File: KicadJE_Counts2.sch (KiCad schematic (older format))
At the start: 91 parts, among them J403 Out 1, J404 In_1, J405 Out 2, J406 In 2, J407 Out 1 Final, J408 Out 2 Final, U401 TL072, U402 TL072

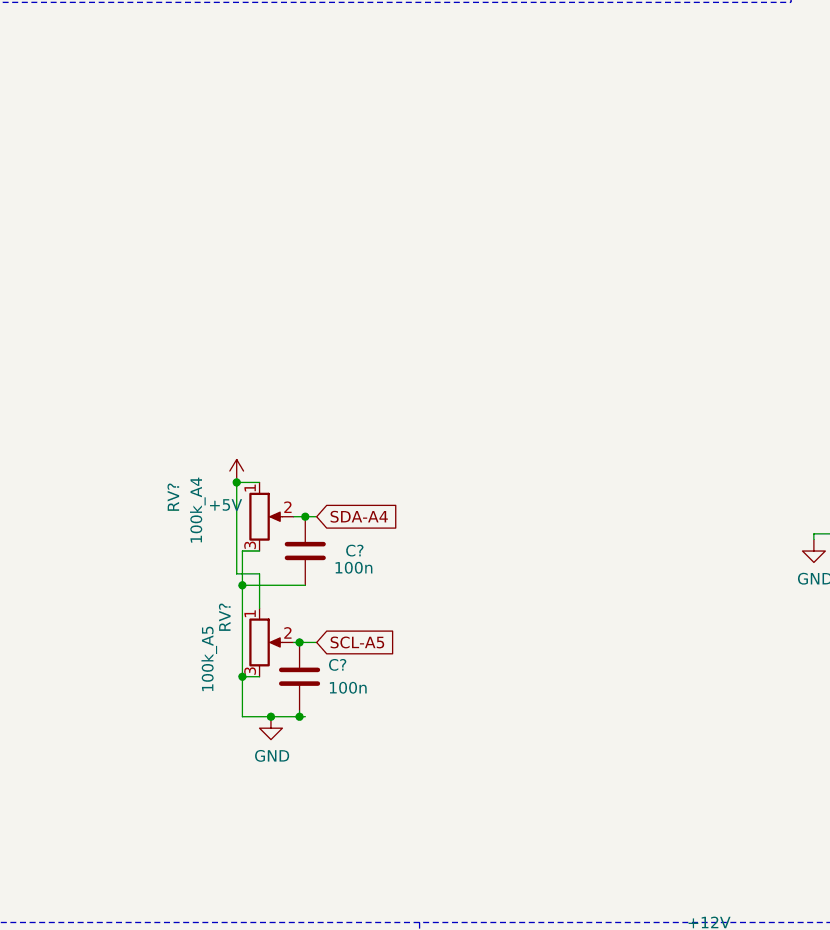
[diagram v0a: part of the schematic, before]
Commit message: Update KicadJE_Counts2.sch
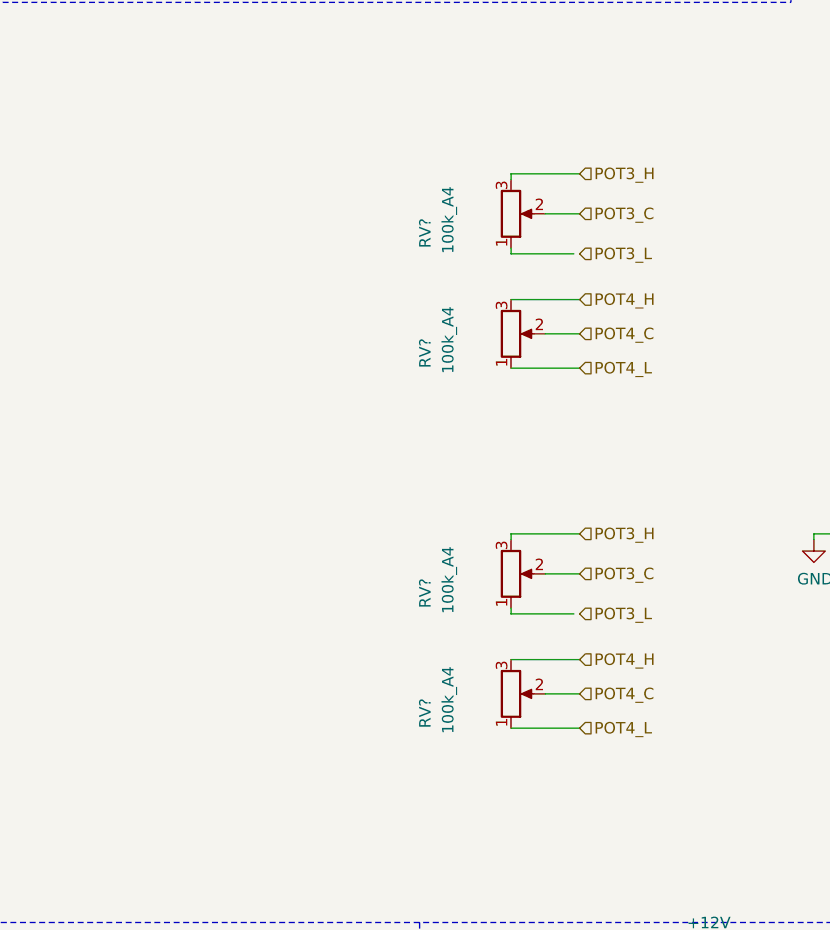
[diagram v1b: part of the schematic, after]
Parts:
- removed C? (x2): 100n, Capacitor_SMD:C_0805_2012Metric_Pad1.15x1.40mm_HandSolder, symbol Device:C
- removed RV?: 100k_A5, Potentiometer_THT:Potentiometer_China_RK09_Single_Vertical_AJ, symbol Device:R_POT
- added RV? (x3): 100k_A4, Potentiometer_THT:Potentiometer_China_RK09_Single_Vertical_AJ, symbol Device:R_POT
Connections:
- net SDA-A4 is gone; now on net POT3_C: RV?.2
- net +5V: no longer RV?.1
- net GND: no longer RV?.3
- net POT3_C: now also RV?.3, RV?.2, RV?.3
- net POT4_C: now also RV?.2, RV?.2, RV?.3, RV?.3
- net POT4_L: now also RV?.1, RV?.1
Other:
- moved on the sheet: RV?
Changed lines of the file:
@@
 Wire Wire Line
 	3800 6100 3875 6100
-Text GLabel 2100 4700 2    50   Input ~ 0
-SCL-A5
-Text GLabel 2100 4150 2    50   Input ~ 0
-SDA-A4
 $Comp
 L Device:R_POT RV?
 U 1 1 5F13A9C4
-P 1850 4150
+P 2950 4400
 AR Path="/5F13A9C4" Ref="RV?"  Part="1"
 AR Path="/5D60ED9A/5F13A9C4" Ref="RV?"  Part="1"
-F 0 "RV?" V 1475 4300 50  0000 R CNN
-F 1 "100k_A4" V 1575 4325 50  0000 R CNN
-F 2 "Potentiometer_THT:Potentiometer_China_RK09_Single_Vertical_AJ" H 1850 4150 50  0001 C CNN
-F 3 "~" H 1850 4150 50  0001 C CNN
-	1    1850 4150
-	1    0    0    -1
-$EndComp
-Wire Wire Line
-	2000 4150 2050 4150
-$Comp
-L Device:R_POT RV?
-U 1 1 5F13A9CB
-P 1850 4700
-AR Path="/5F13A9CB" Ref="RV?"  Part="1"
-AR Path="/5D60ED9A/5F13A9CB" Ref="RV?"  Part="1"
-F 0 "RV?" V 1700 4875 50  0000 R CNN
-F 1 "100k_A5" V 1625 4775 50  0000 R CNN
-F 2 "Potentiometer_THT:Potentiometer_China_RK09_Single_Vertical_AJ" H 1850 4700 50  0001 C CNN
-F 3 "~" H 1850 4700 50  0001 C CNN
-	1    1850 4700
-	1    0    0    -1
-$EndComp
-Wire Wire Line
-	2000 4700 2025 4700
-Wire Wire Line
-	1750 4400 1750 4000
-Wire Wire Line
-	1750 4000 1850 4000
-Wire Wire Line
-	1775 4850 1850 4850
-$Comp
-L power:GND #PWR?
-U 1 1 5F13A9D5
-P 1900 5025
-AR Path="/5F13A9D5" Ref="#PWR?"  Part="1"
-AR Path="/5D60ED9A/5F13A9D5" Ref="#PWR?"  Part="1"
-F 0 "#PWR?" H 1900 4775 50  0001 C CNN
-F 1 "GND" H 1905 4852 50  0000 C CNN
-F 2 "" H 1900 5025 50  0001 C CNN
-F 3 "" H 1900 5025 50  0001 C CNN
-	1    1900 5025
-	1    0    0    -1
-$EndComp
-$Comp
-L power:+5V #PWR?
-U 1 1 5F13A9DB
-P 1750 4000
-AR Path="/5F13A9DB" Ref="#PWR?"  Part="1"
-AR Path="/5D60ED9A/5F13A9DB" Ref="#PWR?"  Part="1"
-F 0 "#PWR?" H 1750 3850 50  0001 C CNN
-F 1 "+5V" H 1700 3900 50  0000 C CNN
-F 2 "" H 1750 4000 50  0001 C CNN
-F 3 "" H 1750 4000 50  0001 C CNN
-	1    1750 4000
-	1    0    0    -1
-$EndComp
-Connection ~ 1750 4000
-$Comp
-L Device:C C?
-U 1 1 5F13A9E2
-P 2025 4850
-AR Path="/5F13A9E2" Ref="C?"  Part="1"
-AR Path="/5D60ED9A/5F13A9E2" Ref="C?"  Part="1"
-F 0 "C?" H 2150 4900 50  0000 L CNN
-F 1 "100n" H 2150 4800 50  0000 L CNN
-F 2 "Capacitor_SMD:C_0805_2012Metric_Pad1.15x1.40mm_HandSolder" H 2063 4700 50  0001 C CNN
-F 3 "~" H 2025 4850 50  0001 C CNN
-	1    2025 4850
-	1    0    0    -1
-$EndComp
-Connection ~ 2025 4700
-Wire Wire Line
-	2025 4700 2100 4700
-Wire Wire Line
-	1775 4850 1775 5025
-Wire Wire Line
-	1775 5025 1900 5025
-Wire Wire Line
-	2025 5025 2025 5000
-Connection ~ 1900 5025
-Wire Wire Line
-	1900 5025 2025 5025
-$Comp
-L Device:C C?
-U 1 1 5F13A9EF
-P 2050 4300
-AR Path="/5F13A9EF" Ref="C?"  Part="1"
-AR Path="/5D60ED9A/5F13A9EF" Ref="C?"  Part="1"
-F 0 "C?" H 2225 4300 50  0000 L CNN
-F 1 "100n" H 2175 4225 50  0000 L CNN
-F 2 "Capacitor_SMD:C_0805_2012Metric_Pad1.15x1.40mm_HandSolder" H 2088 4150 50  0001 C CNN
-F 3 "~" H 2050 4300 50  0001 C CNN
-	1    2050 4300
-	1    0    0    -1
-$EndComp
-Connection ~ 2050 4150
-Wire Wire Line
-	2050 4150 2100 4150
-Wire Wire Line
-	2050 5025 2025 5025
-Connection ~ 2025 5025
-Wire Wire Line
-	1850 4550 1850 4400
-Wire Wire Line
-	1850 4400 1750 4400
-Wire Wire Line
-	1850 4300 1775 4300
-Wire Wire Line
-	1775 4300 1775 4450
-Connection ~ 1775 4850
-Wire Wire Line
-	2050 4450 1775 4450
-Connection ~ 1775 4450
-Wire Wire Line
-	1775 4450 1775 4850
+F 0 "RV?" V 2575 4550 50  0000 R CNN
+F 1 "100k_A4" V 2675 4575 50  0000 R CNN
+F 2 "Potentiometer_THT:Potentiometer_China_RK09_Single_Vertical_AJ" H 2950 4400 50  0001 C CNN
+F 3 "~" H 2950 4400 50  0001 C CNN
+	1    2950 4400
+	1    0    0    1
+$EndComp
 $Comp
 L Device:C C?
@@
 Wire Notes Line
 	600  1900 4175 1900
+Text HLabel 3250 4225 2    50   Input ~ 0
+POT3_H
+Text HLabel 3250 4400 2    50   Input ~ 0
+POT3_C
+Text HLabel 3250 4575 2    50   Input ~ 0
+POT3_L
+Text HLabel 3250 4775 2    50   Input ~ 0
+POT4_H
+Text HLabel 3250 4925 2    50   Input ~ 0
+POT4_C
+Text HLabel 3250 5075 2    50   Input ~ 0
+POT4_L
+$Comp
+L Device:R_POT RV?
+U 1 1 5F31783B
+P 2950 4925
+AR Path="/5F31783B" Ref="RV?"  Part="1"
+AR Path="/5D60ED9A/5F31783B" Ref="RV?"  Part="1"
+F 0 "RV?" V 2575 5075 50  0000 R CNN
+F 1 "100k_A4" V 2675 5100 50  0000 R CNN
+F 2 "Potentiometer_THT:Potentiometer_China_RK09_Single_Vertical_AJ" H 2950 4925 50  0001 C CNN
+F 3 "~" H 2950 4925 50  0001 C CNN
+	1    2950 4925
+	1    0    0    1
+$EndComp
+Wire Wire Line
+	2950 4775 3250 4775
+Wire Wire Line
+	3100 4925 3250 4925
+Wire Wire Line
+	2950 5075 3250 5075
+Wire Wire Line
+	3225 4575 2950 4575
+Wire Wire Line
+	2950 4575 2950 4550
+Wire Wire Line
+	2950 4250 2950 4225
+Wire Wire Line
+	2950 4225 3250 4225
+Wire Wire Line
+	3100 4400 3250 4400
+$Comp
+L Device:R_POT RV?
+U 1 1 5F3F817E
+P 2950 2825
+AR Path="/5F3F817E" Ref="RV?"  Part="1"
+AR Path="/5D60ED9A/5F3F817E" Ref="RV?"  Part="1"
+F 0 "RV?" V 2575 2975 50  0000 R CNN
+F 1 "100k_A4" V 2675 3000 50  0000 R CNN
+F 2 "Potentiometer_THT:Potentiometer_China_RK09_Single_Vertical_AJ" H 2950 2825 50  0001 C CNN
+F 3 "~" H 2950 2825 50  0001 C CNN
+	1    2950 2825
+	1    0    0    1
+$EndComp
+Text HLabel 3250 2650 2    50   Input ~ 0
+POT3_H
+Text HLabel 3250 2825 2    50   Input ~ 0
+POT3_C
+Text HLabel 3250 3000 2    50   Input ~ 0
+POT3_L
+Text HLabel 3250 3200 2    50   Input ~ 0
+POT4_H
+Text HLabel 3250 3350 2    50   Input ~ 0
+POT4_C
+Text HLabel 3250 3500 2    50   Input ~ 0
+POT4_L
+$Comp
+L Device:R_POT RV?
+U 1 1 5F3F818E
+P 2950 3350
+AR Path="/5F3F818E" Ref="RV?"  Part="1"
+AR Path="/5D60ED9A/5F3F818E" Ref="RV?"  Part="1"
+F 0 "RV?" V 2575 3500 50  0000 R CNN
+F 1 "100k_A4" V 2675 3525 50  0000 R CNN
+F 2 "Potentiometer_THT:Potentiometer_China_RK09_Single_Vertical_AJ" H 2950 3350 50  0001 C CNN
+F 3 "~" H 2950 3350 50  0001 C CNN
+	1    2950 3350
+	1    0    0    1
+$EndComp
+Wire Wire Line
+	2950 3200 3250 3200
+Wire Wire Line
+	3100 3350 3250 3350
+Wire Wire Line
+	2950 3500 3250 3500
+Wire Wire Line
+	3225 3000 2950 3000
+Wire Wire Line
+	2950 3000 2950 2975
+Wire Wire Line
+	2950 2675 2950 2650
+Wire Wire Line
+	2950 2650 3250 2650
+Wire Wire Line
+	3100 2825 3250 2825
 $EndSCHEMATC
